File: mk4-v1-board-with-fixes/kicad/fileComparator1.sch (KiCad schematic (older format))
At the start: 4 parts, among them U3 LM339

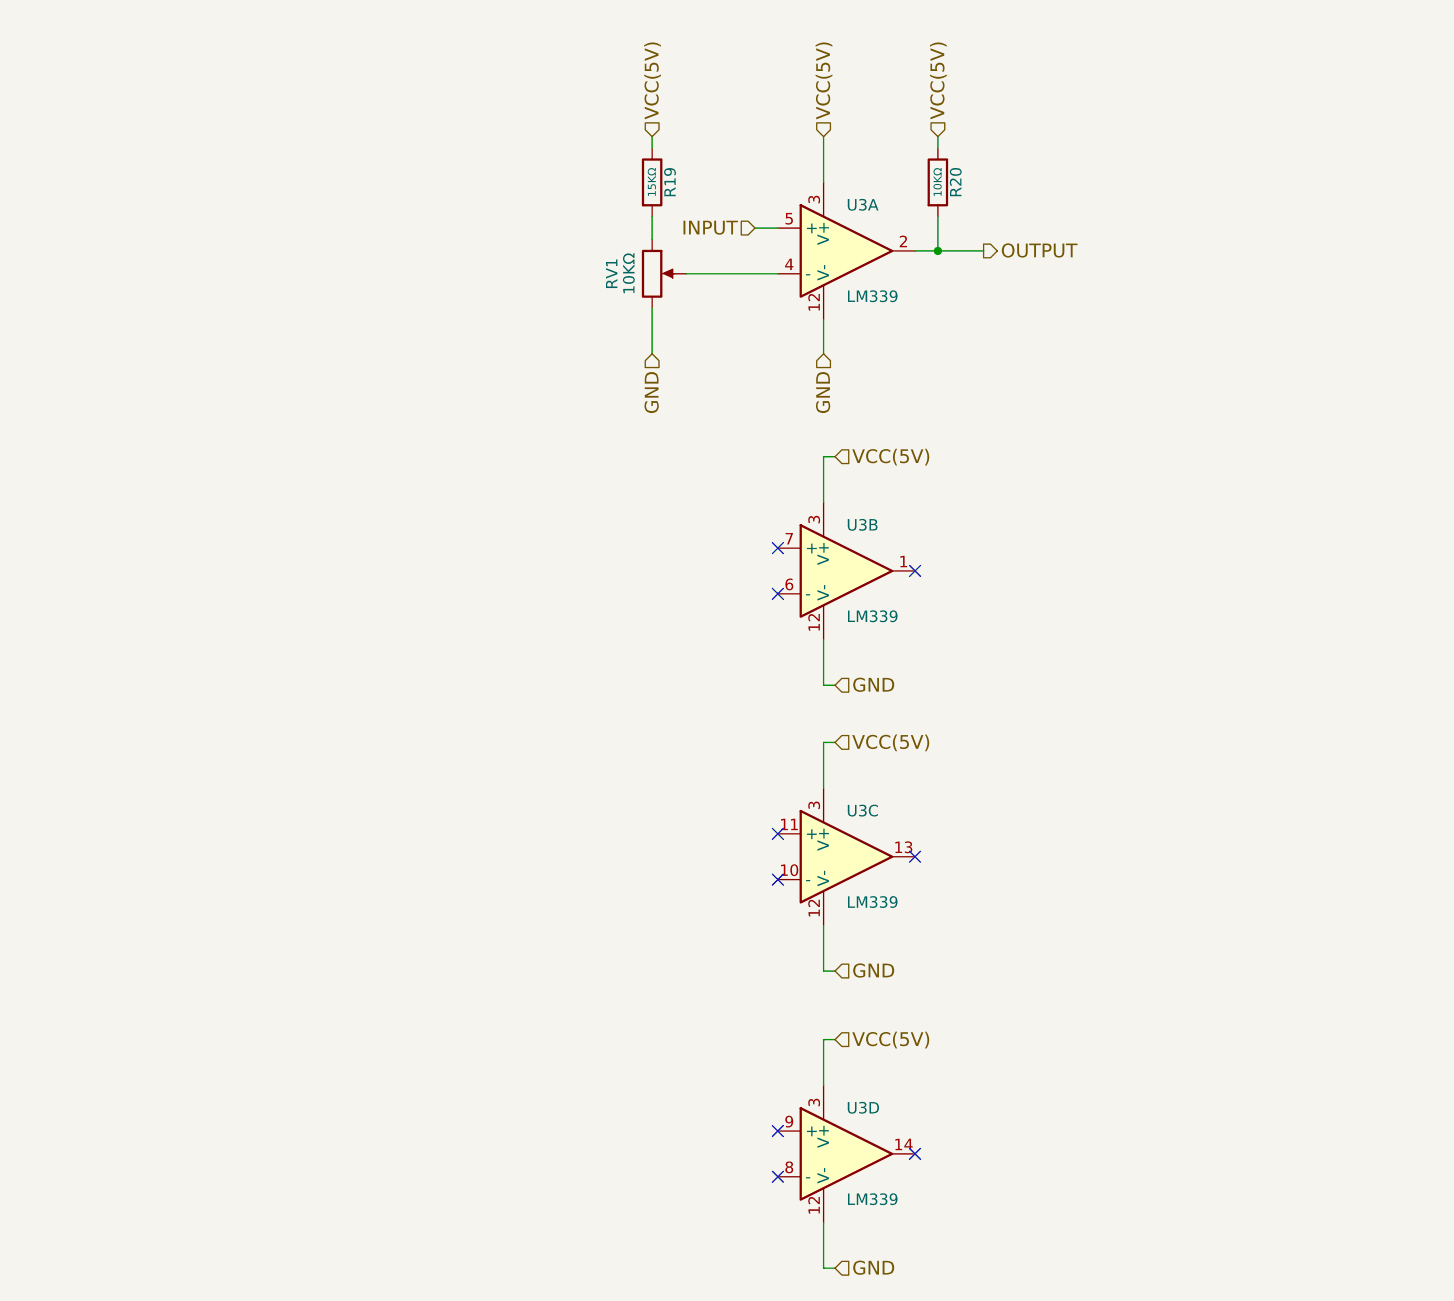
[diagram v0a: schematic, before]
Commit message: Soft push of v2 board modifications
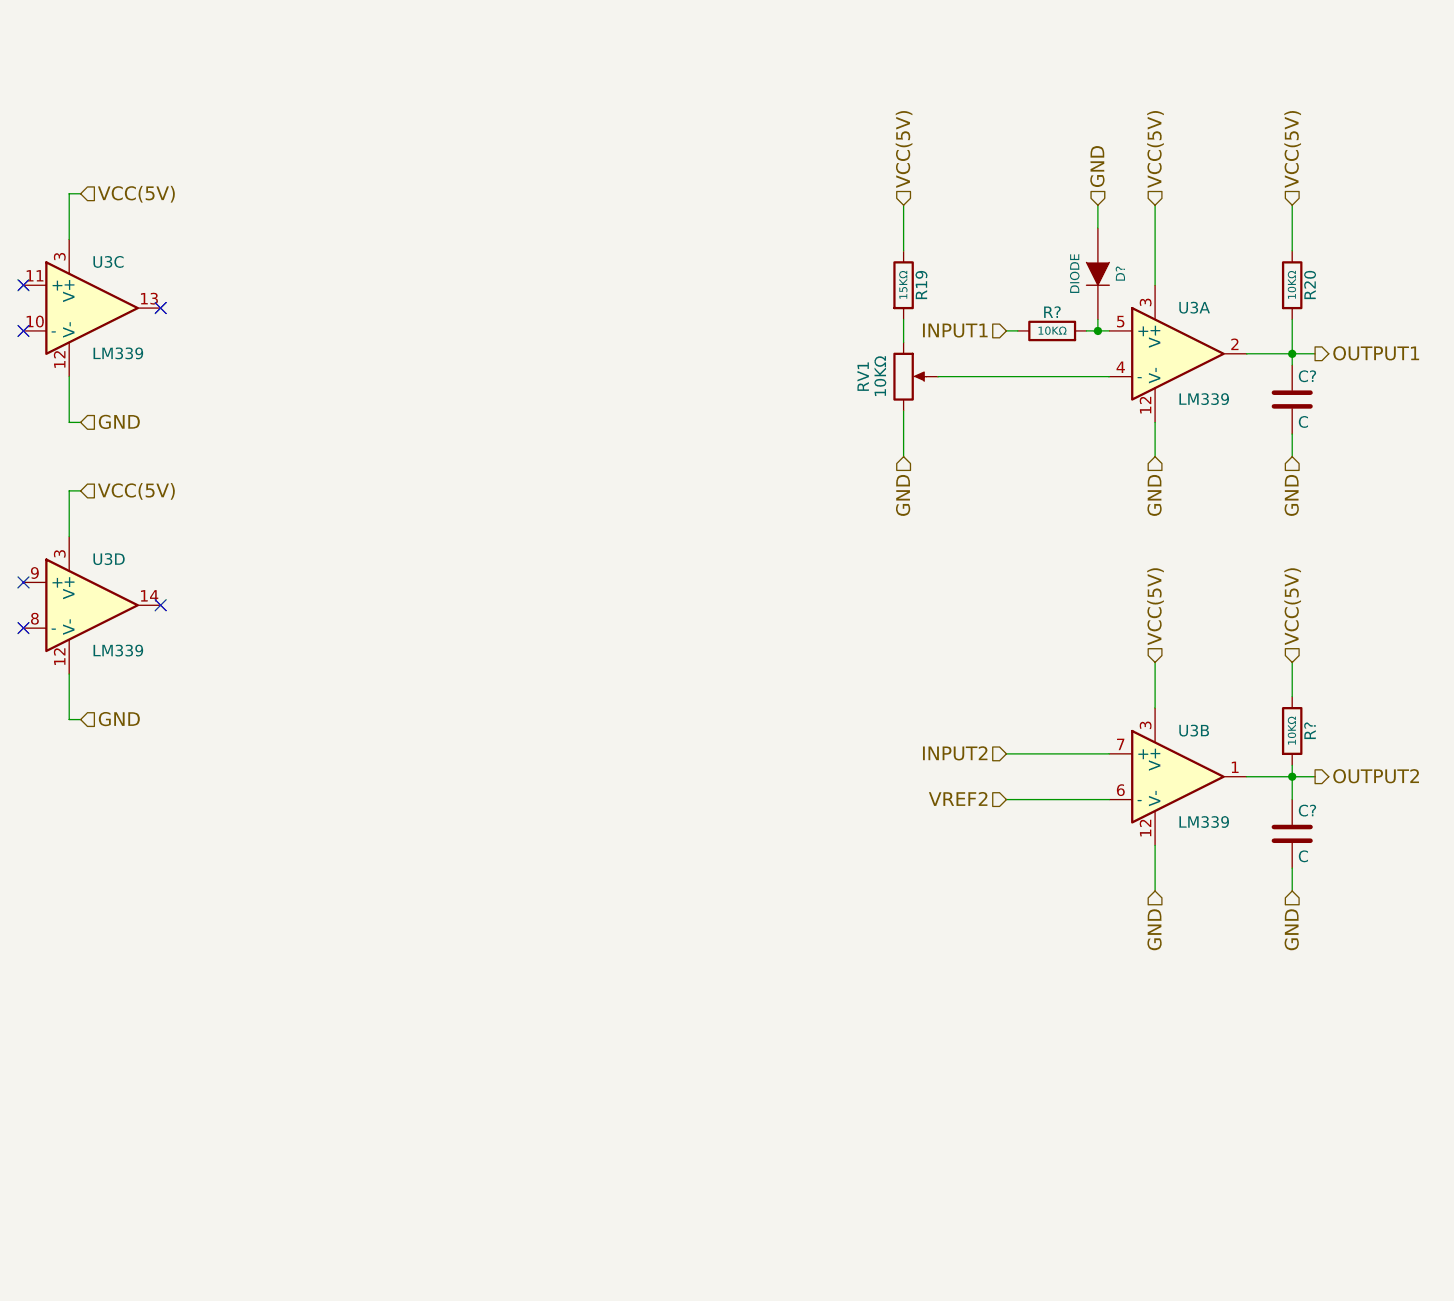
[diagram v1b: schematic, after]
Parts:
- added C? (x2): C, symbol C
- added D?: DIODE, symbol DIODE
- added R? (x2): 10KΩ, Resistors_THT:R_Axial_DIN0207_L6.3mm_D2.5mm_P10.16mm_Horizontal, symbol R
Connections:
- net GND: now also C?.2, C?.2, D?.A
- net VCC(5V): now also R?.1
- net OUTPUT2: now reaches U3.1
- net OUTPUT2: now also C?.1, R?.2
- net VREF2: now reaches U3.6 (-)
- net INPUT2: now reaches U3.7 (+)
- net INPUT: no longer names the net of U3.5 (+)
- net INPUT: now also D?.K, R?.2
- net OUTPUT renamed OUTPUT1
- net OUTPUT1: now also C?.1
- new net INPUT1: R?.1
- no-connect marks 9 -> 6
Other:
- moved on the sheet: R19, R20, RV1, U3A, U3B, U3C, U3D
